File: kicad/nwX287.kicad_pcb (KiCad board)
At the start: 2 copper layers, 18.3 x 31.1 mm, 5 parts, among them J1 Conn_01x03_Male, U1 bq4285, U2 socket, Y1 32.768kHz 6pF

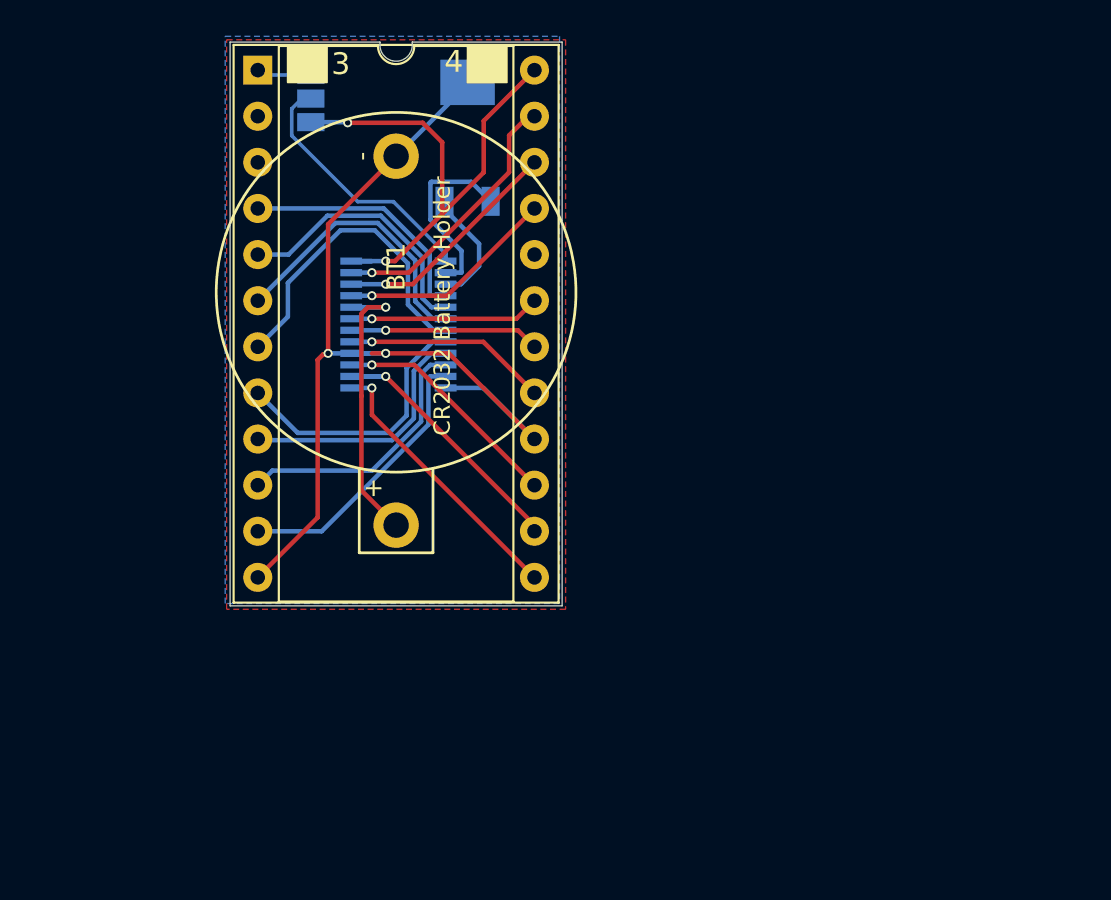
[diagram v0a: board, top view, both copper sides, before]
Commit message: change layout
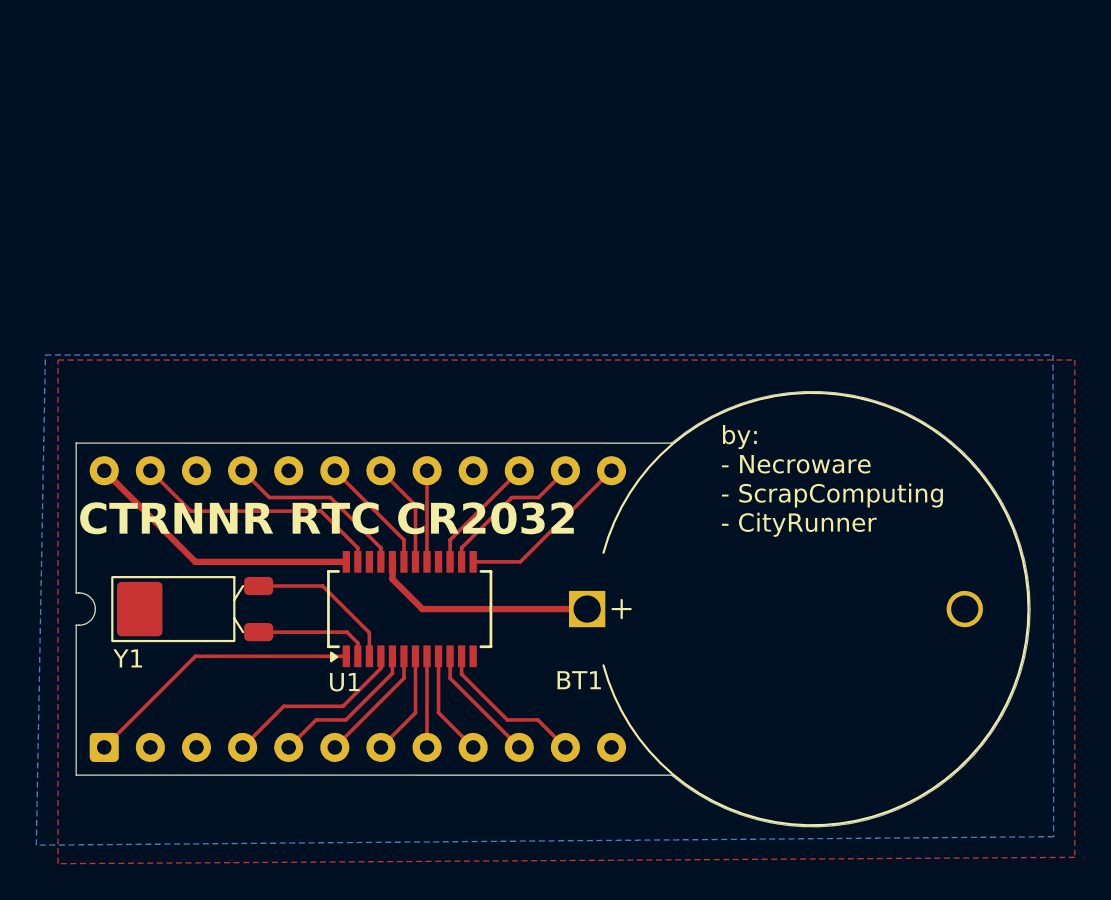
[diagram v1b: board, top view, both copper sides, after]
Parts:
- removed J1: Conn_01x03_Male, Jumper:SolderJumper-3_P1.3mm_Open_Pad1.0x1.5mm_NumberLabels
- BT1: footprint nwX287.2032.ssop:CR2032_battery_holder -> Battery:BatteryHolder_MYOUNG_BS-07-A1BJ001_CR2032
- U1: value bq4285 -> bq3285; moved to F.Cu
- U2: value socket -> Socket
- Y1: moved to F.Cu
- moved U2 38.3 mm to (118.5, 116.8), turned to 90 degrees
- moved Y1 29.9 mm to (123.8, 109.1), turned to -90 degrees
- moved U1 15.7 mm to (135.4, 109.1), turned to 90 degrees
- moved BT1 11.5 mm to (145.1, 109.1), turned to 0 degrees
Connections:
- net CEI renamed RCL
- U1 pad 1: Net-(J1-Pad2) -> MOT
- U1 pad 22: CEO -> unconnected-(U1-NC-Pad22)
- U2 pad 1: VOUT -> MOT
- U2 pad 16: GND -> unconnected-(U2-GND-Pad16)
- U2 pad 2: (no net) -> unconnected-(U2-X1-Pad2)
- U2 pad 20: (no net) -> unconnected-(U2-BC-Pad20)
- U2 pad 22: CEO -> unconnected-(U2-NC-Pad22)
- U2 pad 3: (no net) -> unconnected-(U2-X2-Pad3)
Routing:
- net GND: track 53.7 -> 0.00 mm, vias 2 -> 0
- net MOT: track 0.00 -> 15.4 mm
- net Net-(J1-Pad2): track 14.8 -> 0.00 mm
- net VCC: track 28.9 -> 15.4 mm, vias 2 -> 0
- net CEO: track 13.3 -> 0.00 mm, vias 1 -> 0
- net AD3: track 17.7 -> 5.81 mm
- net AD4: track 14.9 -> 5.02 mm
- net AD2: track 15.6 -> 6.60 mm
- net AD5: track 13.9 -> 5.81 mm
- net AD6: track 14.6 -> 6.60 mm
- net AS: track 15.5 -> 8.25 mm, vias 1 -> 0
- net AD7: track 15.4 -> 8.37 mm
- net AD1: track 14.6 -> 8.34 mm
- net RW: track 12.8 -> 6.60 mm, vias 1 -> 0
- net DS: track 11.3 -> 5.02 mm, vias 1 -> 0
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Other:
- board size 18.3 x 31.1 mm -> 52.5 x 24 mm
- net class Default removed
- net class Power removed
- board text added: "CTRNNR RTC CR2032"
- board text added: "by: - Necroware - ScrapComputing - CityRunner"
- board text removed: "1-2 2-3"
- board text removed: "1-2 N/A"
- board text removed: "2"
- board text removed: "24-SSOP"
- board text removed: "3"
- board text removed: "3287"
- board text removed: "4"
- board text removed: "4287"
- board text removed: "CR2032 Battery Holder"
- board text removed: "Intel Motorola"
- board text removed: "J1(MOT)"
- board text removed: "by Necroware 2032 SSOP by Scrap Computing"
- board text removed: "by Necroware CR2032 SSOP MOT by Scrap Computing"
- board text removed: "nwX287.2032.ssop.mot"
- board text removed: "rev.1a.2032.ssop.mot"
